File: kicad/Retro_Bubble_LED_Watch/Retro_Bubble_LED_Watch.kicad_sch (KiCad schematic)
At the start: 21 parts, among them J1 ISP Programming Connector, SW1 KMS231G, SW2 KMS231G, U1 ATmega328PB-A, U2 DS1337S+

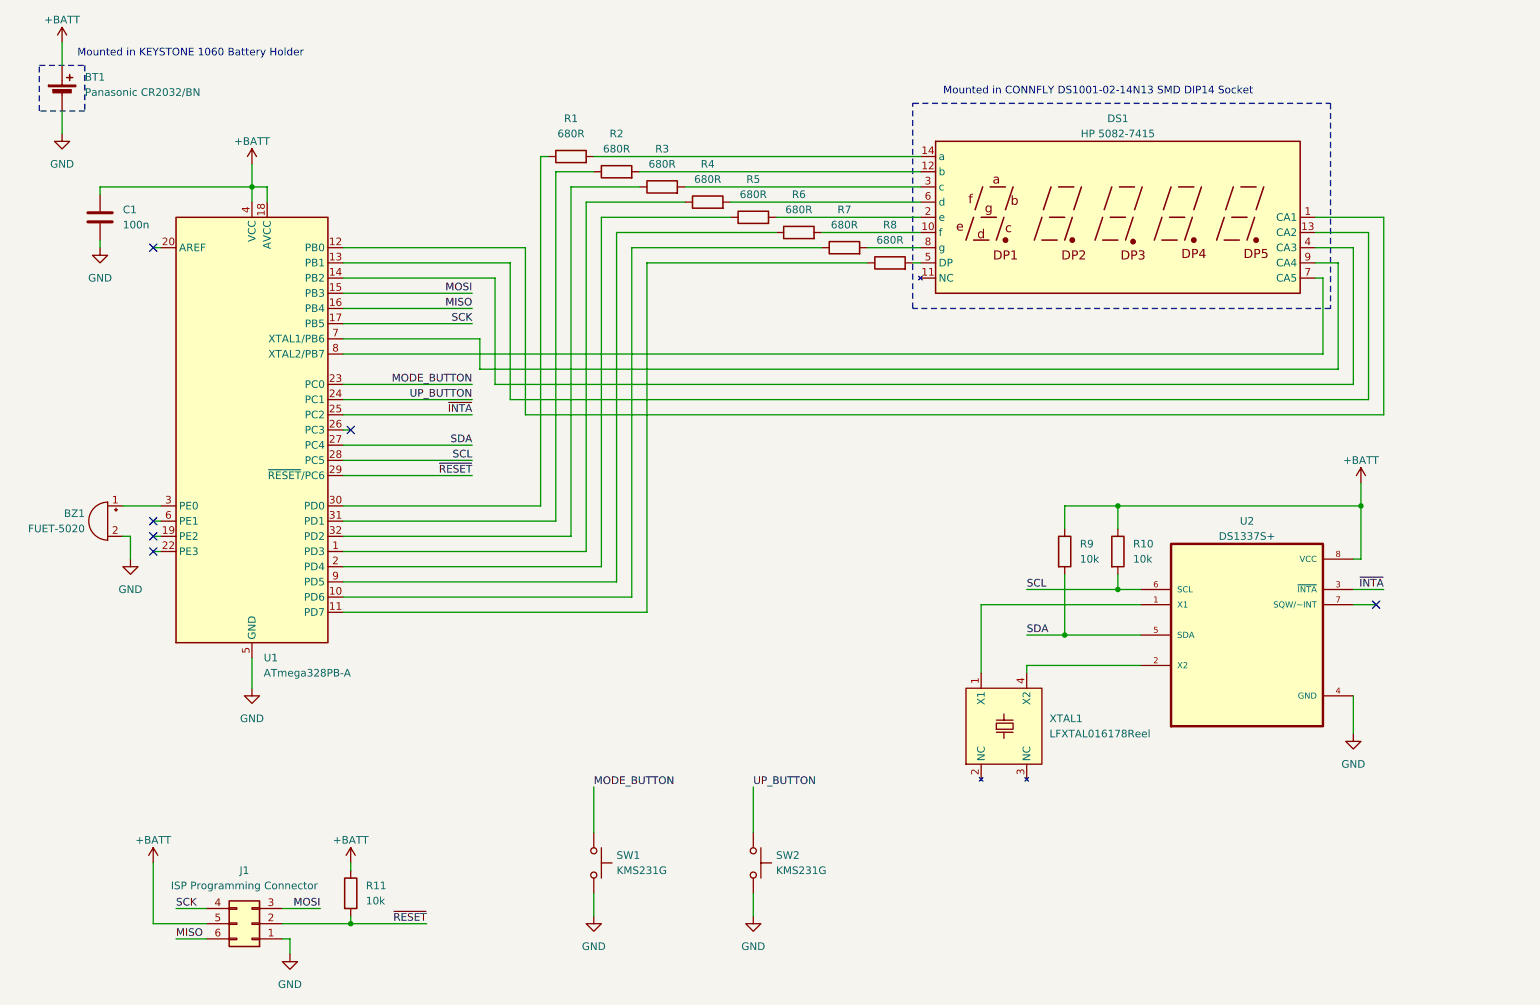
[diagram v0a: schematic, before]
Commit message: Rev. 1.1
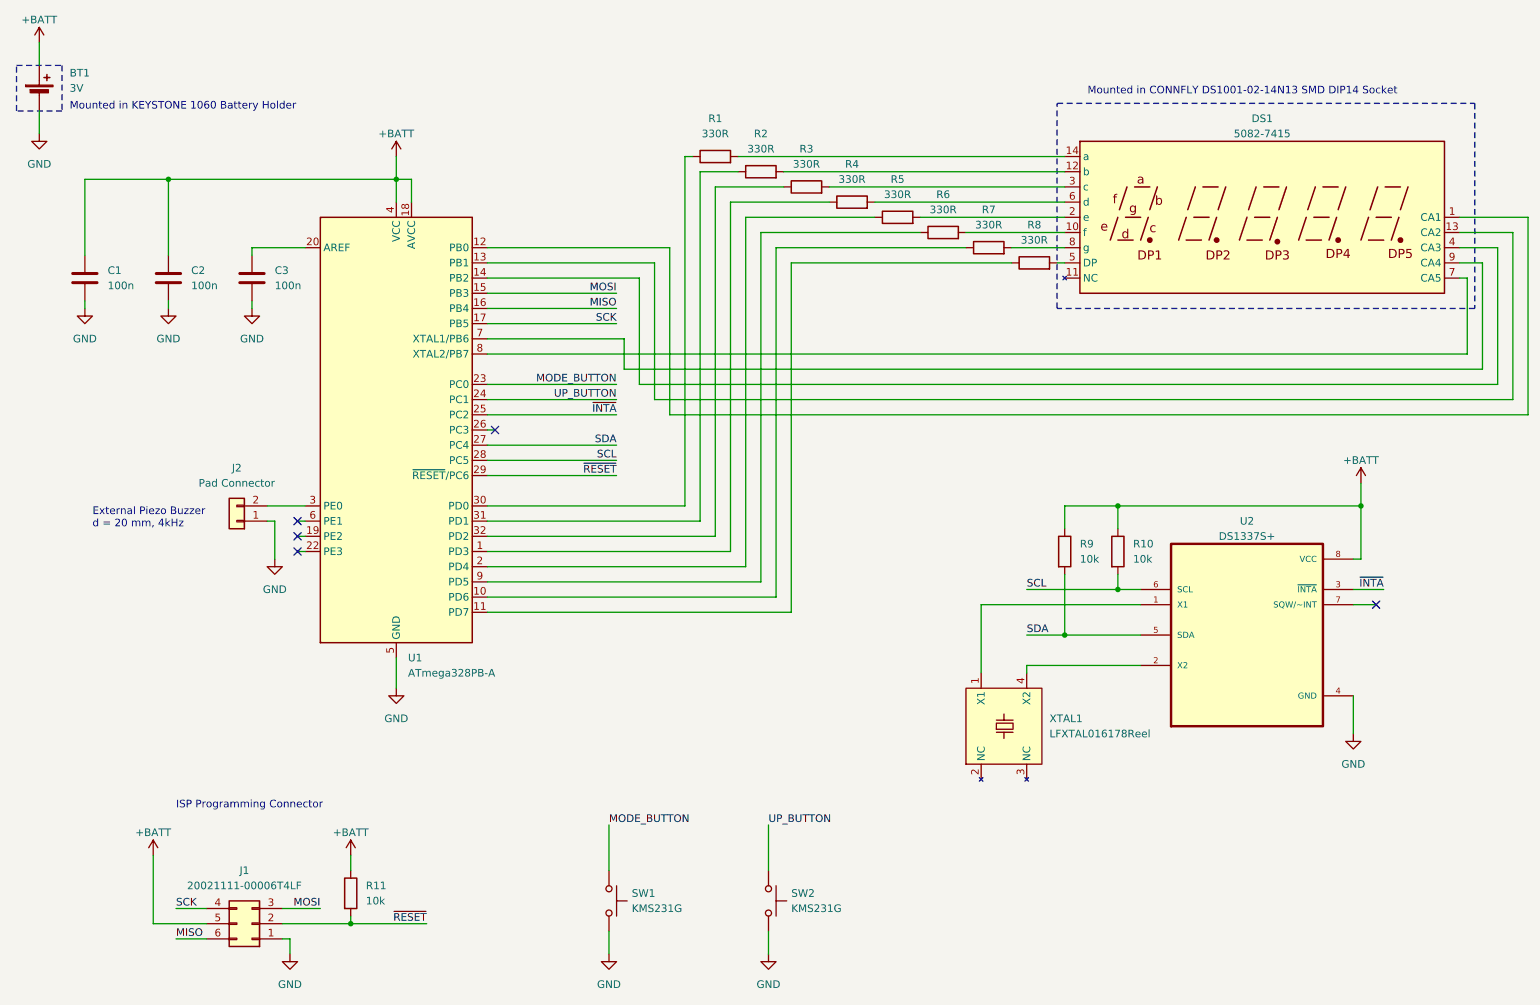
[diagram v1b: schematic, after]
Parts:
- removed BZ1: FUET-5020, footprints:FUET-5020, symbol Device:Buzzer
- added C2, C3: 100n, Capacitor_SMD:C_0603_1608Metric, symbol Device:C
- added J2: Pad Connector, footprints:Pad_Conn_2x1_2x1mm_2.54mm, symbol Connector_Generic:Conn_01x02
- BT1: value Panasonic CR2032/BN -> 3V; footprint Battery:BatteryHolder_Keystone_1058_1x2032 -> Battery:BatteryHolder_Keystone_1060_1x2032; Manufacturer (none) -> PANASONIC; Model (none) -> CR2032/BN; Socket  (none) -> KEYSTONE 1060
- C1: Manufacturer (none) -> SAMSUNG; Model (none) -> CL10B104KA8NFNC
- DS1: value HP 5082-7415 -> 5082-7415; Manufacturer (none) -> HP; Socket (none) -> CONNFLY DS1001-02-14N13
- J1: value ISP Programming Connector -> 20021111-00006T4LF; Manufacturer (none) -> AMPHENOL COMMUNICATIONS SOLUTIONS
- R1, R2, R3, R4, R5, R6, R7, R8: value 680R -> 330R; Manufacturer (none) -> PANASONIC; Model (none) -> ERJ3EKF3300V
- R10, R11, R9: Manufacturer (none) -> PANASONIC; Model (none) -> ERJ3EKF1002V
- SW1, SW2: Manufacturer (none) -> C&K; Model (none) -> KMS231GLFS
- U1: Manufacturer (none) -> MICROCHIP
- U2: Manufacturer (none) -> MAXIM INTEGRATED
- XTAL1: footprint Crystal:Crystal_SMD_SeikoEpson_MC306-4Pin_8.0x3.2mm_HandSoldering -> footprints:LFXTAL016178Reel; Manufacturer (none) -> IQD FREQUENCY PRODUCTS
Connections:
- net +BATT: now also C2.1
- net GND: now also C2.2, C3.2, J2.1 (Pin_1)
- net at U1.20 (AREF): now also C3.1
- net at U1.3 (PE0): now also J2.2 (Pin_2)
- no-connect marks 6 -> 5
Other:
- note added: "External Piezo Buzzer d = 20 mm, 4kHz"
- note added: "ISP Programming Connector"
- moved on the sheet: BT1, C1, DS1, R1, R2, R3, R4, R5, R6, R7, R8, SW1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
